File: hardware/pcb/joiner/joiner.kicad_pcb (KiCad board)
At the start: 2 copper layers, 154 x 70.5 mm, 20 parts, among them J1 XBee3 TH, J2 XBee3 TH, J3 Screw_Terminal_01x02, J4 Screw_Terminal_01x02, K1 1-1393210-3, Q1 2N3904, SW1 SW_Push, U1 ESP32-C3_SUPERMINI_TH, U2 HLK-PM12, U3 HLK-PM01

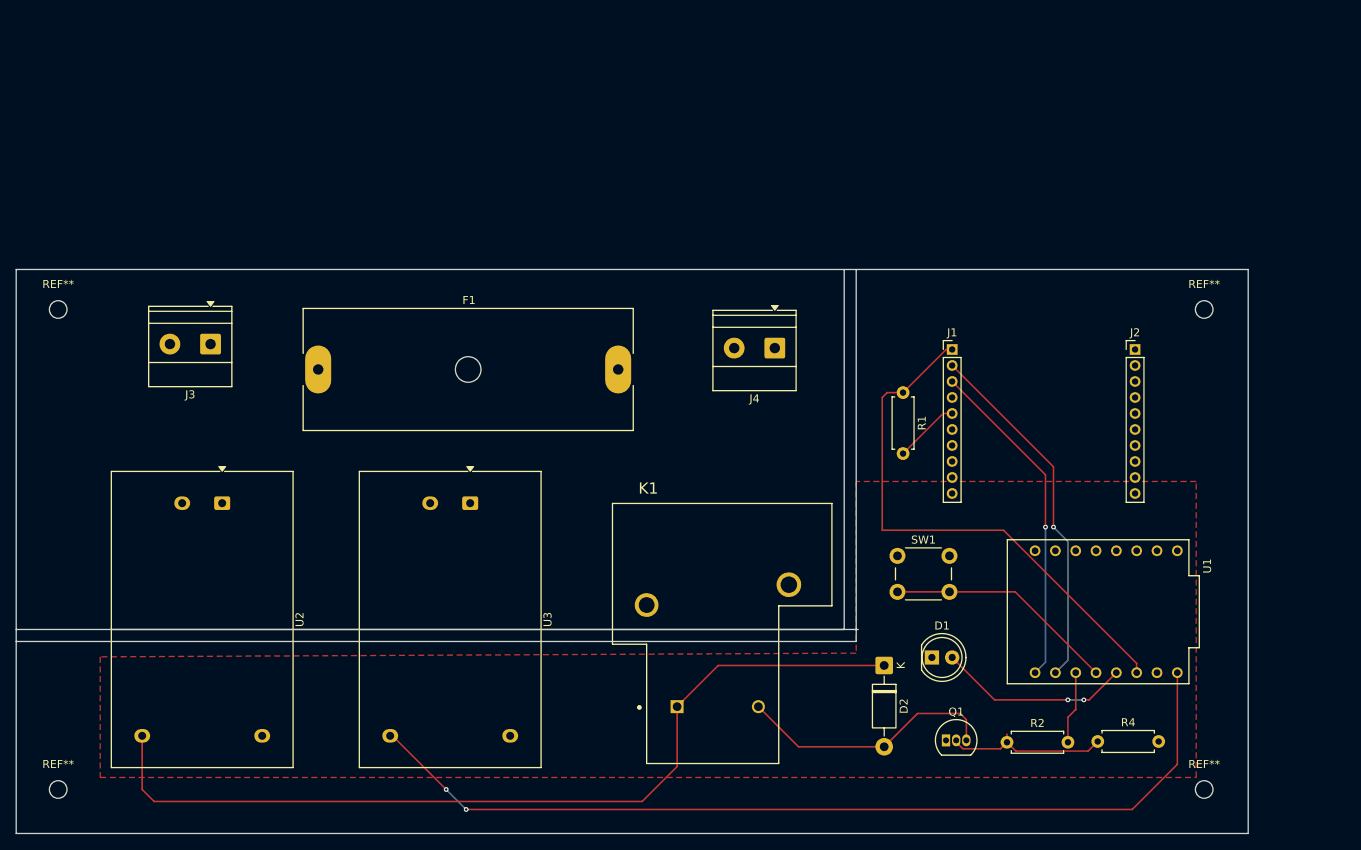
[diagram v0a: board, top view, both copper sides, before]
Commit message: All PCBs finalized, ready to order
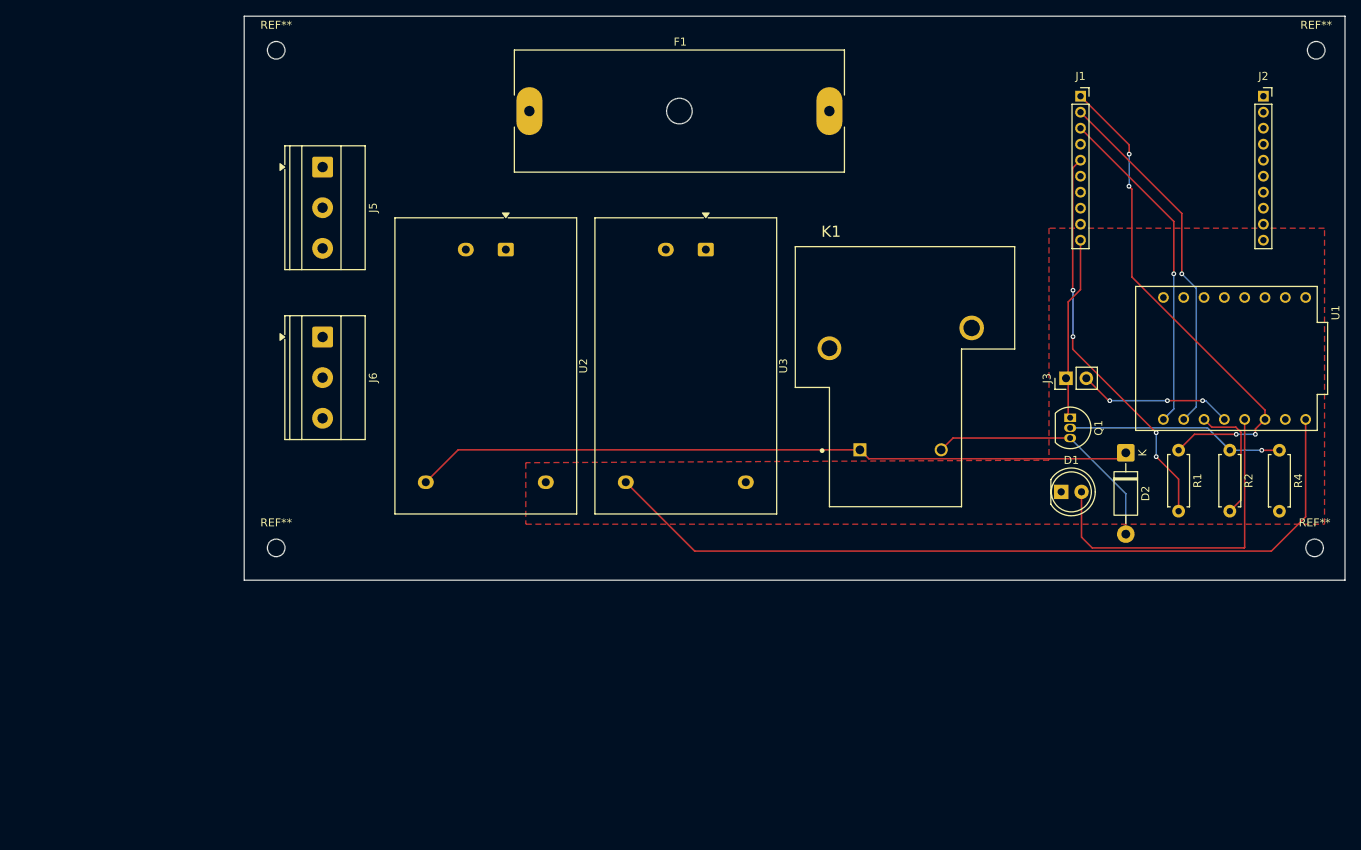
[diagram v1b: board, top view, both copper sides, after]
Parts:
- removed J4: Screw_Terminal_01x02, TerminalBlock_Phoenix:TerminalBlock_Phoenix_MKDS-1,5-2-5.08_1x02_P5.08mm_Horizontal
- removed SW1: SW_Push, Button_Switch_THT:SW_PUSH_6mm
- added J5: Screw_Terminal_01x03, TerminalBlock_Phoenix:TerminalBlock_Phoenix_MKDS-1,5-3-5.08_1x03_P5.08mm_Horizontal, F.Cu at (99.8, 42.2)
- added J6: Screw_Terminal_01x03, TerminalBlock_Phoenix:TerminalBlock_Phoenix_MKDS-1,5-3-5.08_1x03_P5.08mm_Horizontal, F.Cu at (99.8, 63.4)
- F1: value Fuse -> Fuse_15A_SlowBlow
- J1, J2: footprint Connector_PinHeader_2.00mm:PinHeader_1x10_P2.00mm_Vertical -> Connector_PinSocket_2.00mm:PinSocket_1x10_P2.00mm_Vertical
- J3: value Screw_Terminal_01x02 -> Push_Btn; footprint TerminalBlock_Phoenix:TerminalBlock_Phoenix_MKDS-1,5-2-5.08_1x02_P5.08mm_Horizontal -> Connector_PinHeader_2.54mm:PinHeader_1x02_P2.54mm_Vertical
- moved J3 107.0 mm to (192.7, 68.6), turned to 90 degrees
- moved U2 47.6 mm to (122.7, 52.5)
- moved R2 45.9 mm to (213.2, 77.6), turned to -90 degrees
- moved U3 43.3 mm to (147.7, 52.5)
- moved Q1 43.2 mm to (193.2, 73.5), turned to -90 degrees
- moved R4 42.9 mm to (219.4, 77.6), turned to -90 degrees
- moved REF** 42.3 mm to (94.0, 27.6)
- moved F1 41.7 mm to (125.7, 35.2)
- moved REF** 40.7 mm to (94.0, 89.8)
- moved D2 40.2 mm to (200.2, 77.9)
- moved K1 39.4 mm to (167.0, 77.5)
- moved J1 35.5 mm to (194.5, 33.3)
- moved J2 35.5 mm to (217.4, 33.3)
- moved U1 35.5 mm to (212.8, 66.1)
- moved REF** 35.3 mm to (224.0, 27.6)
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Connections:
- F1 pad 1: Net-(J3-Pin_2) -> Net-(J5-Pin_3)
- J3 pad 1: Net-(J3-Pin_1) -> GND
- U1 pad 3: Net-(U1-GPIO3) -> Net-(J3-Pin_2)
- U2 pad 2: Net-(J3-Pin_1) -> Net-(J5-Pin_2)
- U3 pad 2: Net-(J3-Pin_1) -> Net-(J5-Pin_2)
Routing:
- net Net-(J1-RST): track 8.22 -> 49.8 mm, vias 0 -> 4
- net Net-(U1-GPIO3): track 29.0 -> 0.00 mm
- net GND: track 0.00 -> 22.9 mm
- net Net-(D2-K): track 111.5 -> 89.9 mm
- net Net-(J3-Pin_2): track 0.00 -> 19.6 mm, vias 0 -> 3
- net Net-(D1-A): track 24.1 -> 42.6 mm, vias 2 -> 0
- net Net-(U3-+Vout): track 116.0 -> 102.5 mm, vias 2 -> 0
- net Net-(Q1-B): track 20.6 -> 27.3 mm, vias 0 -> 1
- net Net-(U1-GPIO2): track 9.16 -> 15.7 mm
- net +3.3V: track 67.7 -> 62.8 mm, vias 0 -> 4
- net Net-(D2-A): track 32.7 -> 31.7 mm
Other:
- board size 154 x 70.5 mm -> 137.6 x 70.5 mm
- board text added: "137.6mm x 70.5mm"
- board text removed: "Slot_Cut"
